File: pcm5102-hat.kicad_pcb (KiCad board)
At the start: 2 copper layers, 46.7 x 51.8 mm, 2 parts, among them J1 GPIO

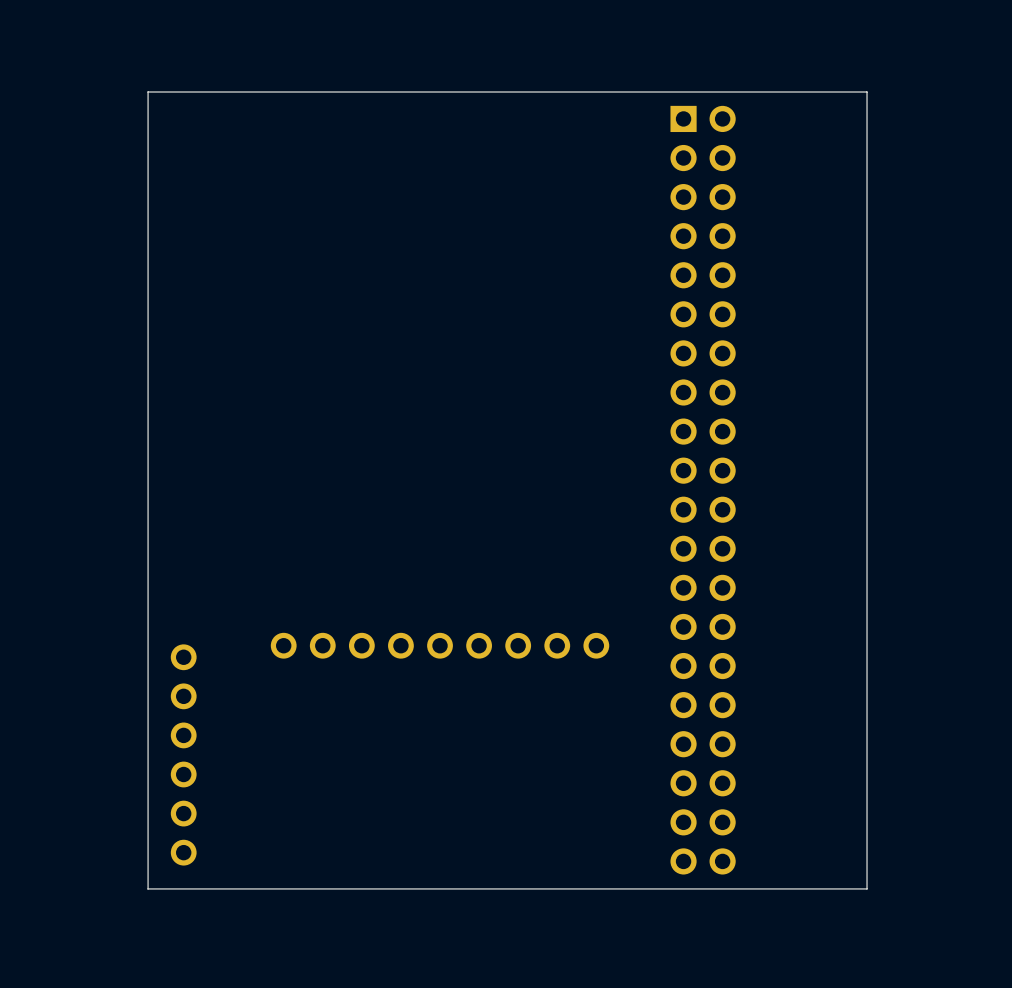
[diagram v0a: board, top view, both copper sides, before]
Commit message: finish routing
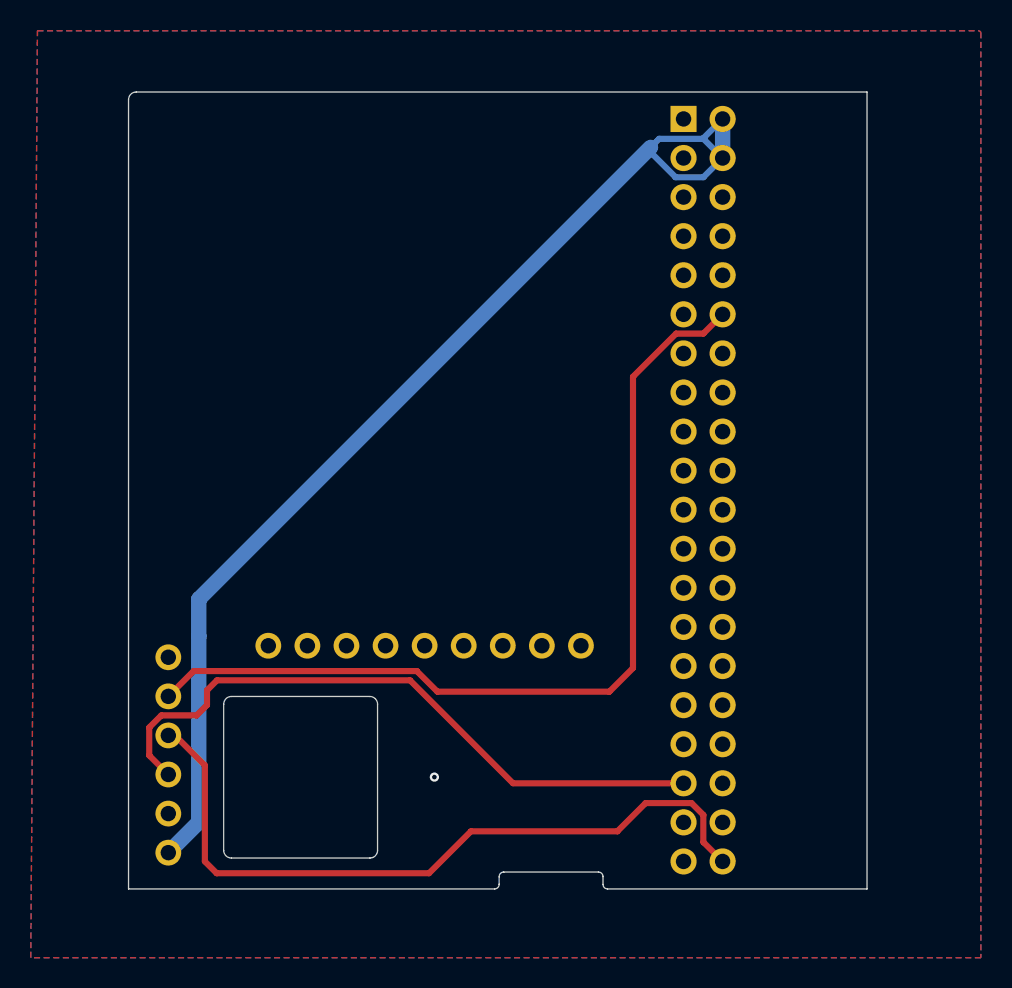
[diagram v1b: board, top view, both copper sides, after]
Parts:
- moved U1 1.00 mm to (90.6, 95.5)
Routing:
- net +5V: track 0.00 -> 74.8 mm
- net BCK: track 0.00 -> 58.5 mm
- net DIN: track 0.00 -> 47.9 mm
- net LCK: track 0.00 -> 42.9 mm
- net GND: vias 0 -> 1
- added copper zone on B.Cu, net GND
- added copper zone on F.Cu, net GND
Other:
- board size 46.7 x 51.8 mm -> 48 x 51.8 mm
